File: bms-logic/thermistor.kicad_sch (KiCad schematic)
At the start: 2 parts, among them P1 SM02B-NSHSS-TB_LF_SN

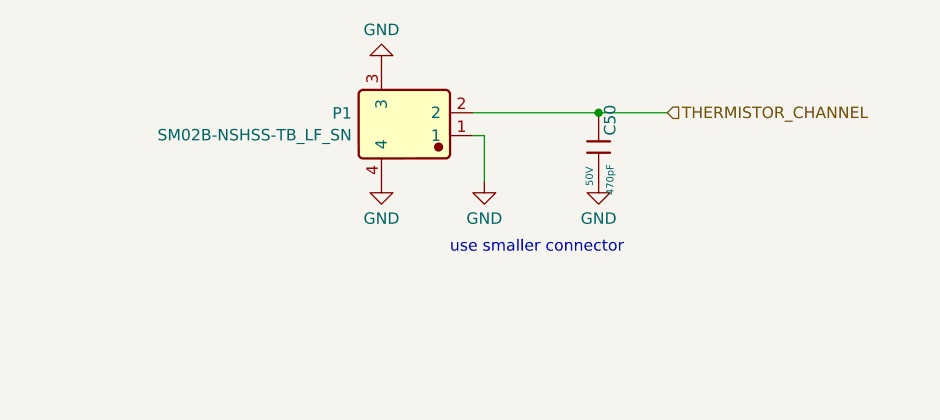
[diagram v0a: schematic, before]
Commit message: diagonal
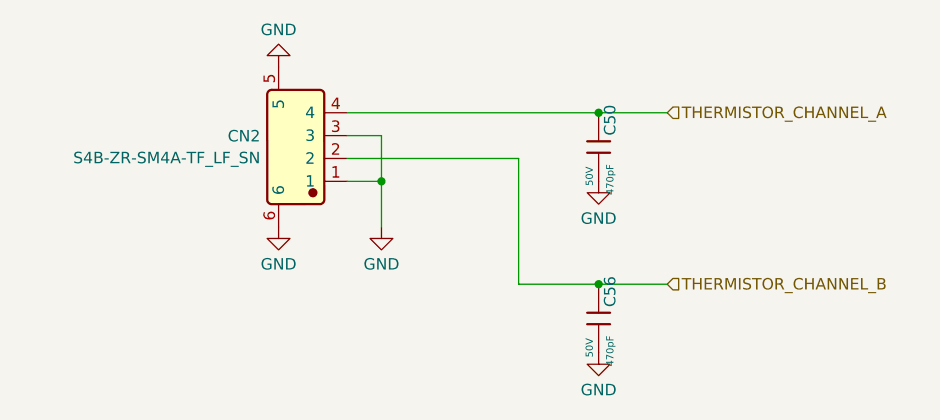
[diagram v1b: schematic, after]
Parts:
- removed P1: SM02B-NSHSS-TB_LF_SN, JLCImport:SM02B-NSHSS-TB_LF_SN, symbol JLCImport:SM02B-NSHSS-TB_LF_SN
- added C56: 470pF, PCM_JLCPCB:C_0402, symbol PCM_JLCPCB-Capacitors:0402,470pF
- added CN2: S4B-ZR-SM4A-TF_LF_SN, JLCImport:JST_ZH_S4B-ZR-SM4A-TF_1x04-1MP_P1.50mm_Horizontal, symbol JLCImport:S4B-ZR-SM4A-TF_LF_SN
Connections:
- net GND: now also C56.2, CN2.1, CN2.3, CN2.5, CN2.6
- net THERMISTOR_CHANNEL renamed THERMISTOR_CHANNEL_A
- net THERMISTOR_CHANNEL_A: now also CN2.4
- new net THERMISTOR_CHANNEL_B: C56.1, CN2.2
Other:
- note removed: "use smaller connector"
